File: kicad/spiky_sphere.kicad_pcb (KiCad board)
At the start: 2 copper layers, 101.6 x 66 mm, 139 parts, among them K1 CONN_3, K2 CONN_3, K3 CONN_3, K4 CONN_3, K5 CONN_3, K6 CONN_3, K7 CONN_3, P1 CONN_8, U1 LED_MTX_5X7

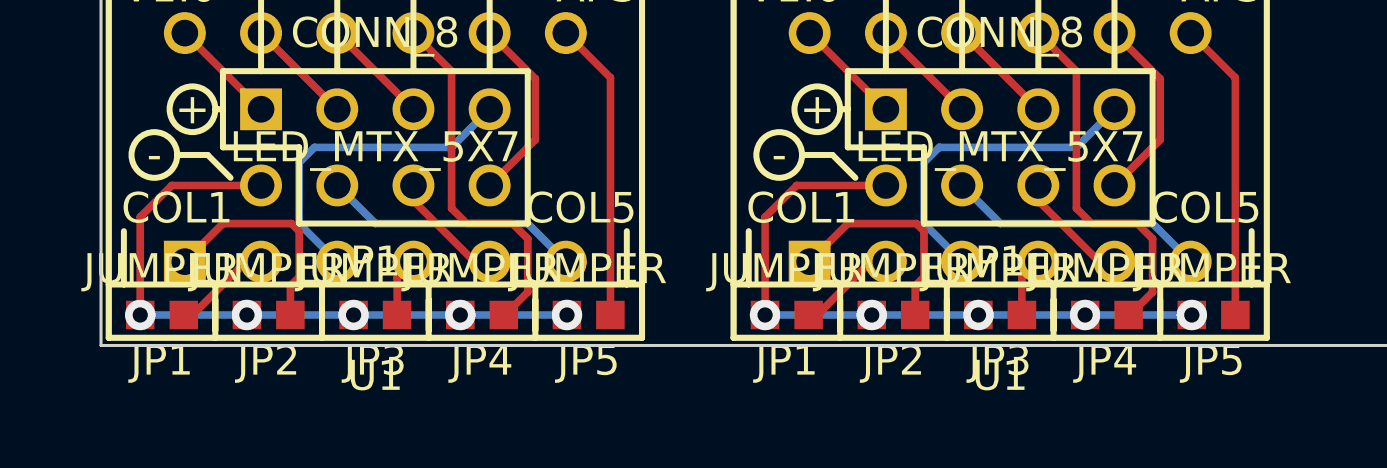
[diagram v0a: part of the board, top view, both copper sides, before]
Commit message: revised files... drill file glitch?
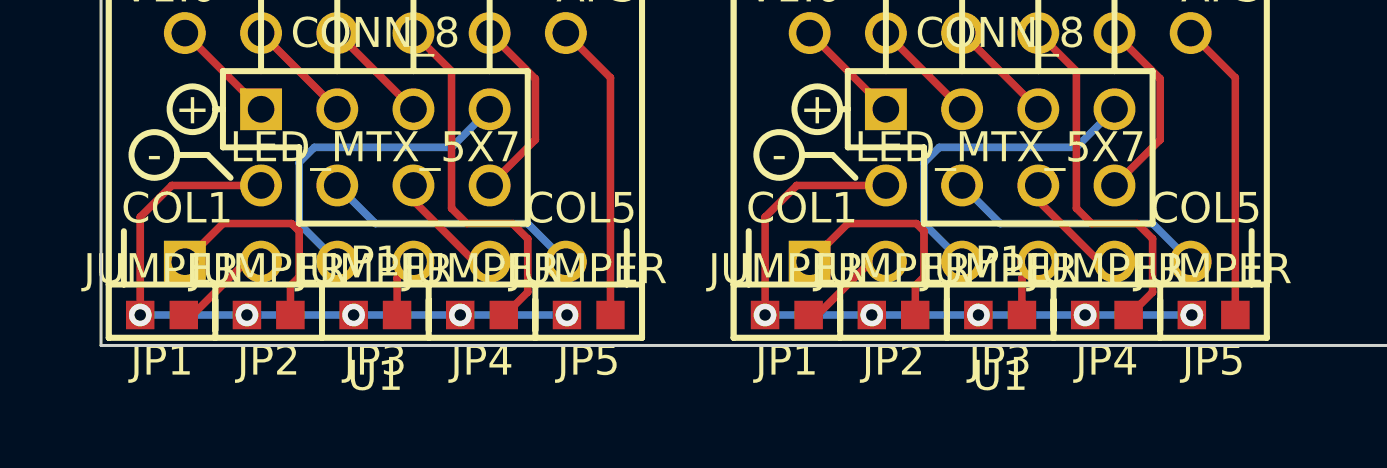
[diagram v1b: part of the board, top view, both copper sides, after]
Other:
- net class Default: via_dia 1.016 -> 0.762; via_drill 0.635 -> 0.381
- rule via_min_drill: 0.508 -> 0.381
- rule via_min_size: 0.889 -> 0.762
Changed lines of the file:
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@@
     (segment_width 0.2)
     (edge_width 0.1)
-    (via_size 1.016)
-    (via_drill 0.635)
-    (via_min_size 0.889)
-    (via_min_drill 0.508)
+    (via_size 0.762)
+    (via_drill 0.381)
+    (via_min_size 0.762)
+    (via_min_drill 0.381)
     (uvia_size 0.508)
     (uvia_drill 0.127)
@@
     (clearance 0.254)
     (trace_width 0.254)
-    (via_dia 1.016)
-    (via_drill 0.635)
+    (via_dia 0.762)
+    (via_drill 0.381)
     (uvia_dia 0.508)
     (uvia_drill 0.127)
@@
   (segment (start 115.57 108.204) (end 119.126 108.204) (width 0.254) (layer B.Cu) (net 20))
   (segment (start 112.051 108.204) (end 115.57 108.204) (width 0.254) (layer B.Cu) (net 20))
-  (via (at 112.051 108.204) (size 1.016) (layers F.Cu B.Cu) (net 20))
+  (via (at 112.051 108.204) (size 0.762) (layers F.Cu B.Cu) (net 20))
   (segment (start 126.275 108.204) (end 126.238 108.204) (width 0.254) (layer B.Cu) (net 20))
-  (via (at 126.275 108.204) (size 1.016) (layers F.Cu B.Cu) (net 20))
+  (via (at 126.275 108.204) (size 0.762) (layers F.Cu B.Cu) (net 20))
   (segment (start 122.719 108.204) (end 122.682 108.204) (width 0.254) (layer B.Cu) (net 20))
-  (via (at 122.719 108.204) (size 1.016) (layers F.Cu B.Cu) (net 20))
+  (via (at 122.719 108.204) (size 0.762) (layers F.Cu B.Cu) (net 20))
   (segment (start 119.163 108.204) (end 119.126 108.204) (width 0.254) (layer B.Cu) (net 20))
-  (via (at 119.163 108.204) (size 1.016) (layers F.Cu B.Cu) (net 20))
+  (via (at 119.163 108.204) (size 0.762) (layers F.Cu B.Cu) (net 20))
   (segment (start 115.607 108.204) (end 115.57 108.204) (width 0.254) (layer B.Cu) (net 20))
-  (via (at 115.607 108.204) (size 1.016) (layers F.Cu B.Cu) (net 20))
+  (via (at 115.607 108.204) (size 0.762) (layers F.Cu B.Cu) (net 20))
   (segment (start 113.104 103.886) (end 116.078 103.886) (width 0.254) (layer F.Cu) (net 20))
   (segment (start 112.051 104.939) (end 113.104 103.886) (width 0.254) (layer F.Cu) (net 20))
@@
   (segment (start 91.223 104.939) (end 92.276 103.886) (width 0.254) (layer F.Cu) (net 20))
   (segment (start 92.276 103.886) (end 95.25 103.886) (width 0.254) (layer F.Cu) (net 20))
-  (via (at 94.779 108.204) (size 1.016) (layers F.Cu B.Cu) (net 20))
+  (via (at 94.779 108.204) (size 0.762) (layers F.Cu B.Cu) (net 20))
   (segment (start 94.779 108.204) (end 94.742 108.204) (width 0.254) (layer B.Cu) (net 20))
-  (via (at 98.335 108.204) (size 1.016) (layers F.Cu B.Cu) (net 20))
+  (via (at 98.335 108.204) (size 0.762) (layers F.Cu B.Cu) (net 20))
   (segment (start 98.335 108.204) (end 98.298 108.204) (width 0.254) (layer B.Cu) (net 20))
-  (via (at 101.891 108.204) (size 1.016) (layers F.Cu B.Cu) (net 20))
+  (via (at 101.891 108.204) (size 0.762) (layers F.Cu B.Cu) (net 20))
   (segment (start 101.891 108.204) (end 101.854 108.204) (width 0.254) (layer B.Cu) (net 20))
-  (via (at 105.447 108.204) (size 1.016) (layers F.Cu B.Cu) (net 20))
+  (via (at 105.447 108.204) (size 0.762) (layers F.Cu B.Cu) (net 20))
   (segment (start 105.447 108.204) (end 105.41 108.204) (width 0.254) (layer B.Cu) (net 20))
-  (via (at 91.223 108.204) (size 1.016) (layers F.Cu B.Cu) (net 20))
+  (via (at 91.223 108.204) (size 0.762) (layers F.Cu B.Cu) (net 20))
   (segment (start 91.223 108.204) (end 94.742 108.204) (width 0.254) (layer B.Cu) (net 20))
   (segment (start 94.742 108.204) (end 98.298 108.204) (width 0.254) (layer B.Cu) (net 20))
